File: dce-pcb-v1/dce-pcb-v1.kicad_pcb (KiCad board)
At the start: 2 copper layers, 42 parts, among them J1 Conn_01x05_Socket, M1 2N7000, Q1 BC557B, Q10 BC547B, Q11 BC547B, Q2 BC557B, Q3 BC547B, Q4 BC547B, Q5 TIP42C, Q6 TIP41C, Q7 BC547B, U5 LM324, U7 LM324

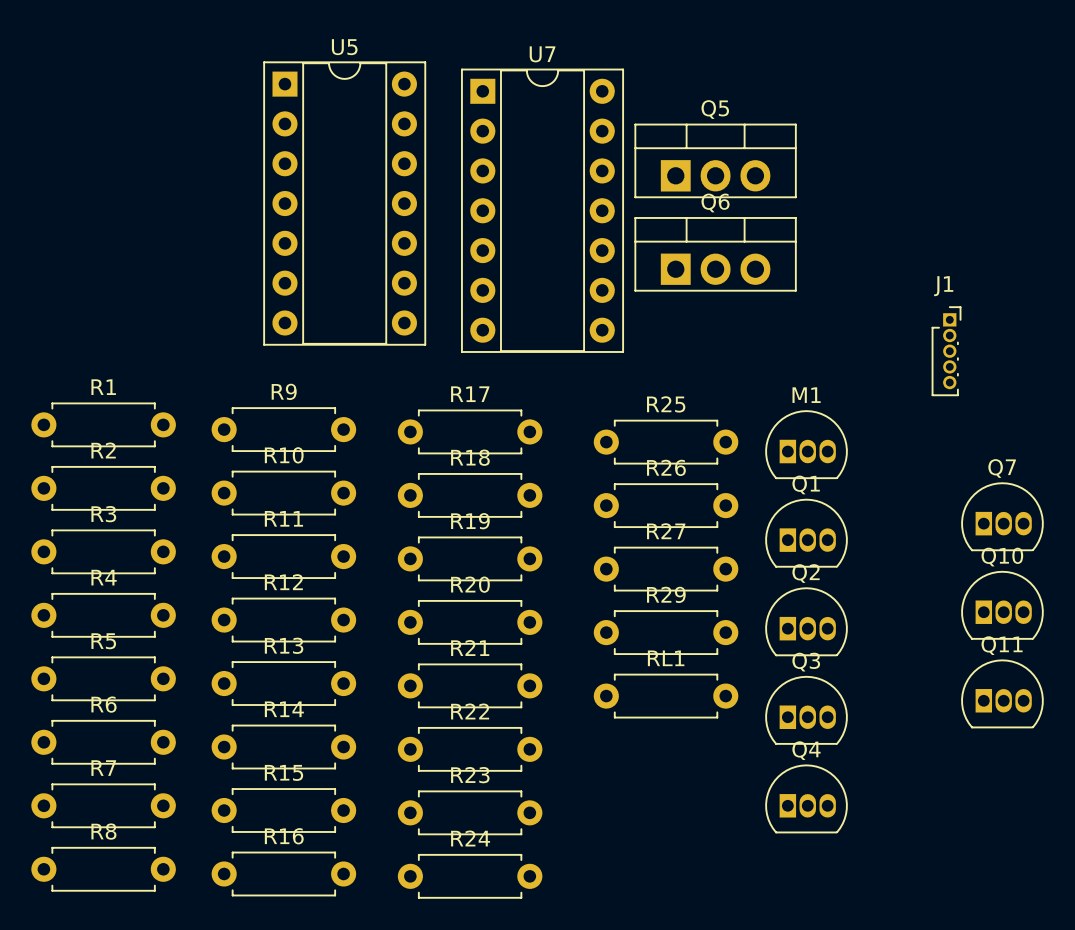
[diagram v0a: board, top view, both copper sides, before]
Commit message: actualiza el pcb
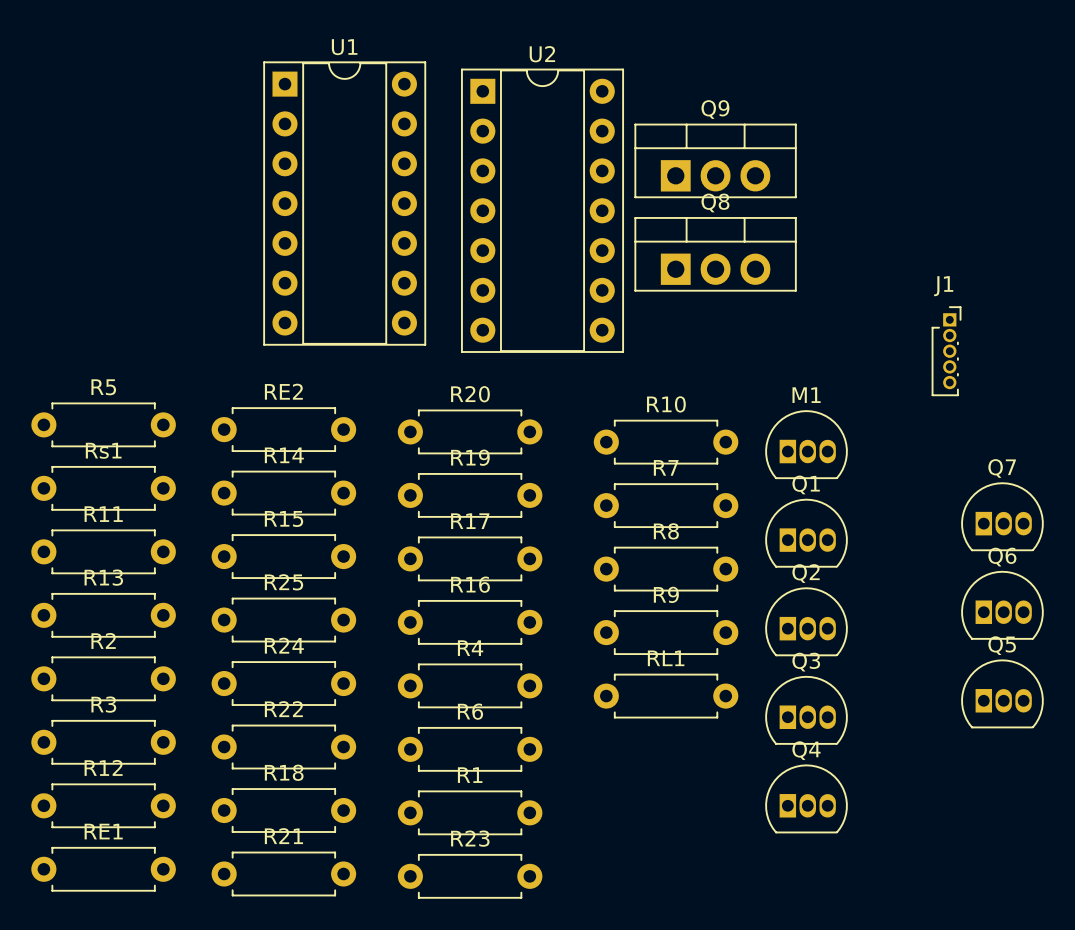
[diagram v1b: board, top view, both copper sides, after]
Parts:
- renumbered Q11 to Q5, Q10 to Q6, Q6 to Q8, Q5 to Q9, R23 to R1, R25 to R10, R3 to R11, R7 to R12, R4 to R13, R10 to R14, R11 to R15, R20 to R16, R19 to R17, R15 to R18, R18 to R19, R5 to R2, R17 to R20, R16 to R21, R14 to R22, R24 to R23, R13 to R24, R12 to R25, R6 to R3, R21 to R4, R1 to R5, R22 to R6, R26 to R7, R27 to R8, R29 to R9, R8 to RE1, R9 to RE2, R2 to Rs1, U5 to U1, U7 to U2
